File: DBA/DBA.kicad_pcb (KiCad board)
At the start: 2 copper layers, 45.7 x 61 mm, 3 parts, among them U1 ESP32_NodeMCU_v1.1

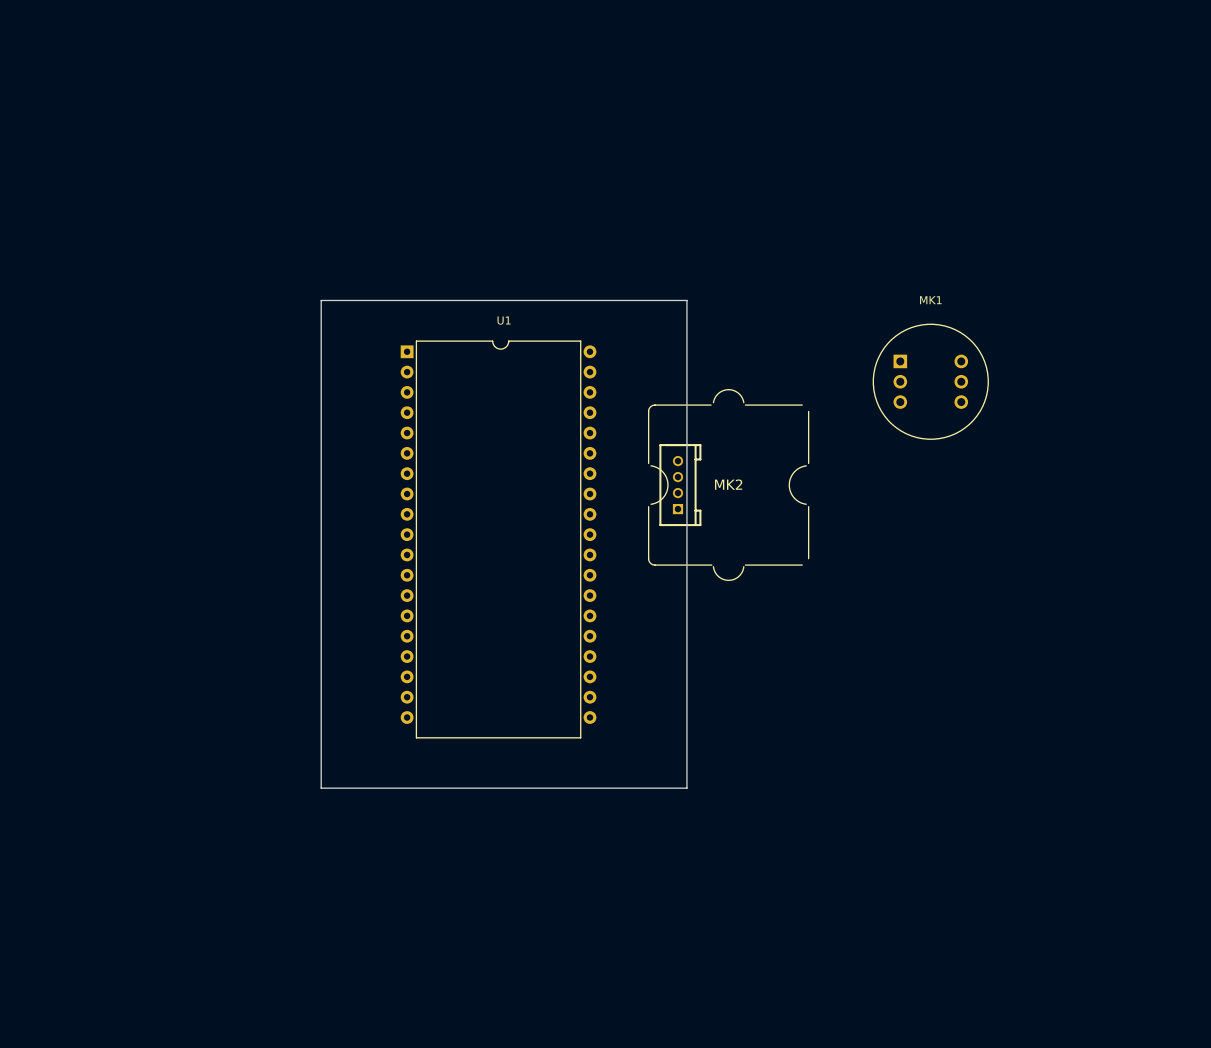
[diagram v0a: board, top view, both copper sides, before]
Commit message: First complete model
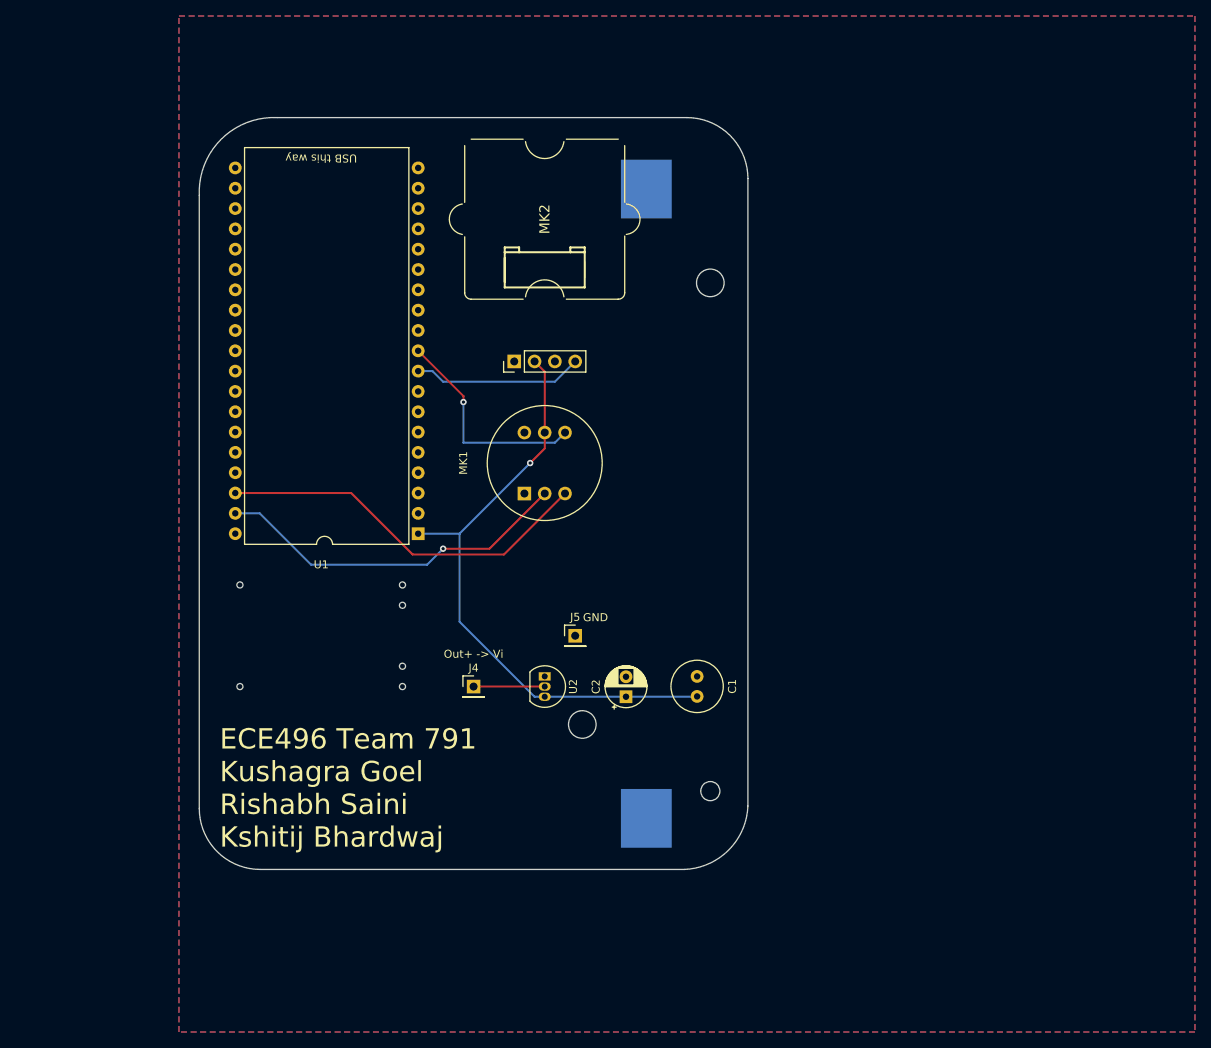
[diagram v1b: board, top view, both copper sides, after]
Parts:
- added A1: TP4056, custom:TP4056Board, B.Cu at (119.4, 101.6)
- added BT1: Battery_Cell, Battery:BatteryHolder_Keystone_1042_1x18650, B.Cu at (160.0, 86.4)
- added C1: 100n, Capacitor_THT:C_Radial_D6.3mm_H5.0mm_P2.50mm, F.Cu at (166.4, 108.0)
- added C2: 100u, Capacitor_THT:CP_Radial_D5.0mm_P2.50mm, F.Cu at (157.5, 110.5)
- added J4: Conn_01x01_Male, Connector_PinHeader_2.54mm:PinHeader_1x01_P2.54mm_Vertical, F.Cu at (138.4, 109.2)
- added J5: Conn_01x01_Male, Connector_PinHeader_2.54mm:PinHeader_1x01_P2.54mm_Vertical, F.Cu at (151.1, 102.9)
- added U2: MCP1700-3302E_TO92, Package_TO_SOT_THT:TO-92_Inline, F.Cu at (147.3, 108.0)
- moved MK1 49.3 mm to (147.3, 81.3), turned to 90 degrees
- moved MK2 40.4 mm to (147.3, 50.8), turned to 90 degrees
- moved U1 30.6 mm to (119.4, 68.6), turned to 180 degrees
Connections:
- MK2 pad 4: unconnected-(MK2-Pad4) -> Net-(MK2-Pad4)
- U1 pad 9: unconnected-(U1-Pad9) -> Net-(MK2-Pad4)
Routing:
- net Net-(C1-Pad2): track 0.00 -> 76.2 mm, vias 0 -> 1
- net Net-(MK1-Pad3): track 0.00 -> 47.6 mm
- net Net-(MK1-Pad2): track 0.00 -> 45.0 mm, vias 0 -> 1
- net Net-(MK1-Pad4): track 0.00 -> 27.1 mm, vias 0 -> 1
- net Net-(MK2-Pad4): track 0.00 -> 21.2 mm
- net Net-(U2-Pad2): track 0.00 -> 8.89 mm
- added copper zone on B.Cu, net GND
- added copper zone on F.Cu, net GND
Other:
- board size 45.7 x 61 mm -> 68.6 x 94 mm
- board text added: "ECE496 Team 791 Kushagra Goel Rishabh Saini Kshitij Bhardwaj"

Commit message: first circular version{
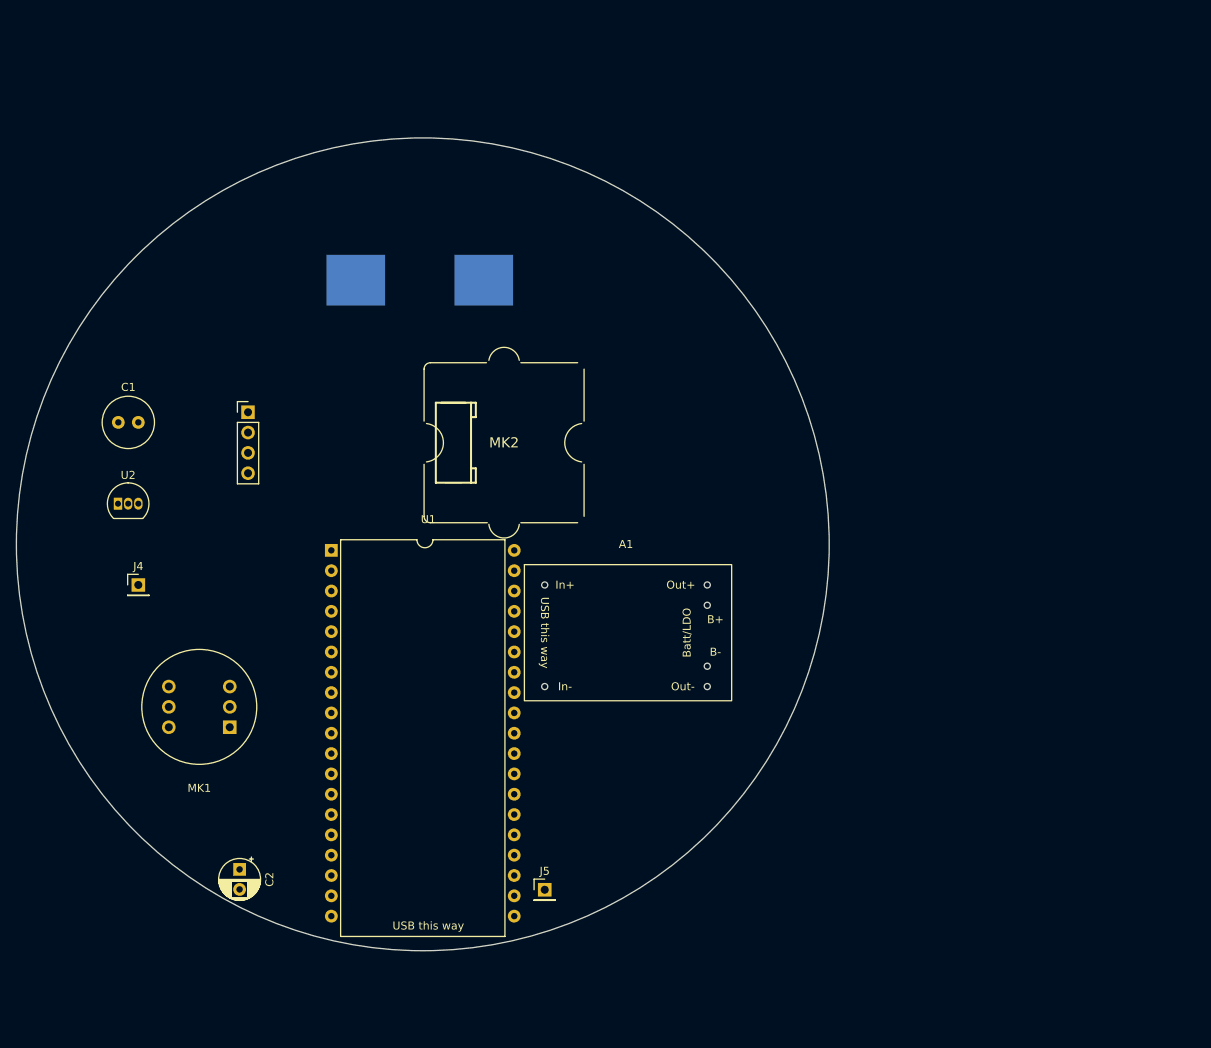
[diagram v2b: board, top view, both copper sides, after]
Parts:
- A1: moved to F.Cu
- BT1: footprint Battery:BatteryHolder_Keystone_1042_1x18650 -> Battery:Battery_Custom
- moved C1 79.0 mm to (94.0, 76.2), turned to 0 degrees
- moved U2 57.5 mm to (94.0, 86.4), turned to 0 degrees
- moved C2 52.9 mm to (109.2, 132.1), turned to -90 degrees
- moved MK1 52.9 mm to (104.1, 111.8), turned to 180 degrees
- moved U1 47.1 mm to (132.8, 113.7), turned to 0 degrees
- moved J4 43.8 mm to (96.5, 96.5)
- moved BT1 40.6 mm to (130.6, 58.4), turned to 180 degrees
- moved A1 38.2 mm to (157.5, 104.1)
- moved J5 32.0 mm to (147.3, 134.6)
- moved MK2 28.4 mm to (142.2, 78.7), turned to 0 degrees
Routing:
- net Net-(C1-Pad2): track 76.2 -> 0.00 mm, vias 1 -> 0
- net Net-(MK1-Pad3): track 47.6 -> 0.00 mm
- net Net-(MK1-Pad2): track 45.0 -> 0.00 mm, vias 1 -> 0
- net Net-(MK1-Pad4): track 27.1 -> 0.00 mm, vias 1 -> 0
- net Net-(MK2-Pad4): track 21.2 -> 0.00 mm
- net Net-(J4-Pad1): track 8.89 -> 0.00 mm
- removed copper zone on B.Cu, net GND
- removed copper zone on F.Cu, net GND
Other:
- board size 68.6 x 94 mm -> 101.6 x 101.6 mm
- board text removed: "ECE496 Team 791 Kushagra Goel Rishabh Saini Kshitij Bhardwaj"

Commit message: Final circular design
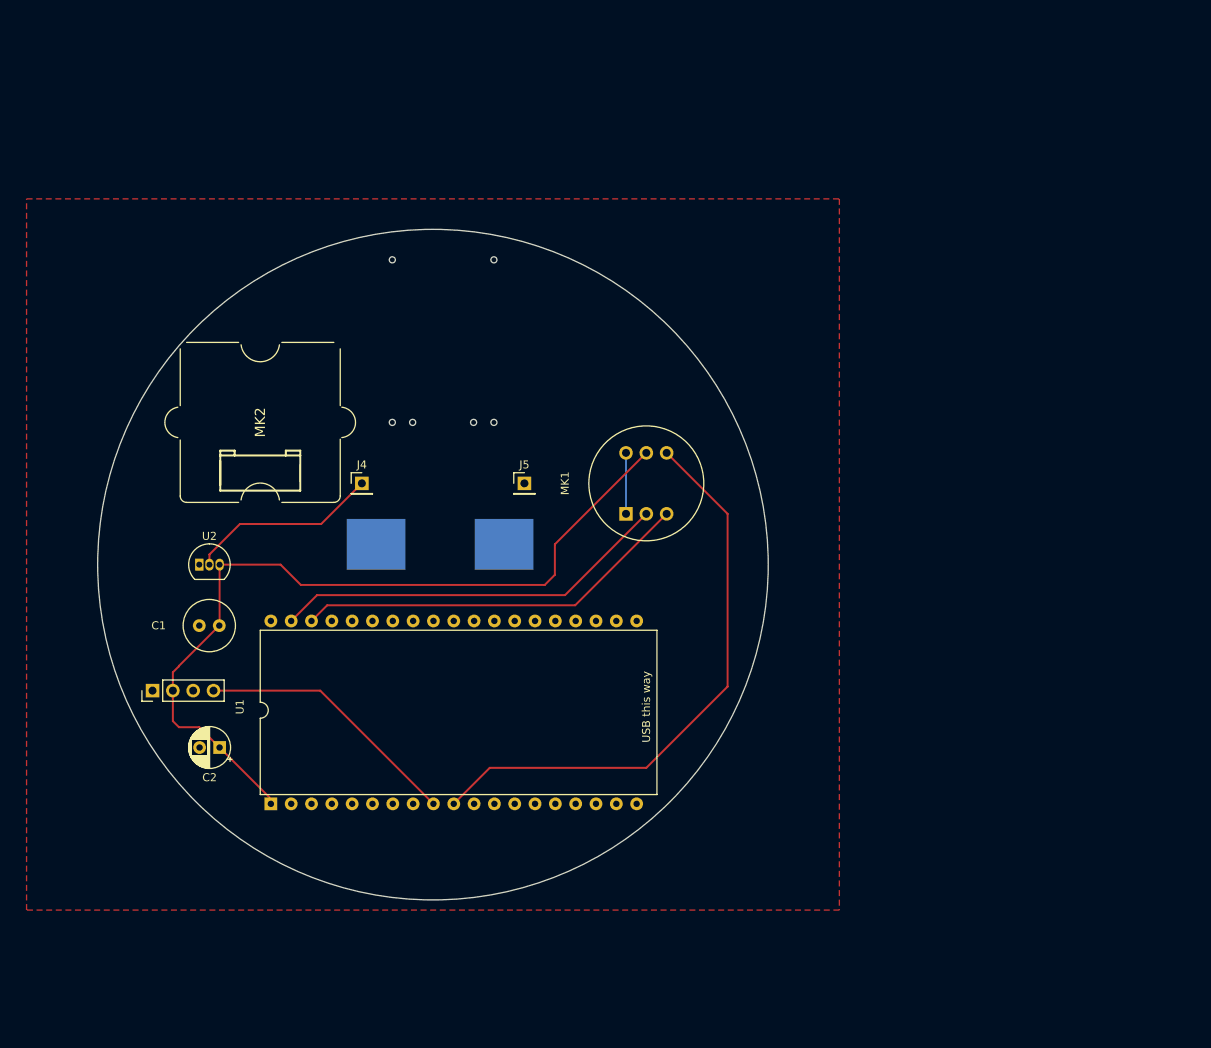
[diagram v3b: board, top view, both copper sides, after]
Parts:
- A1: moved to B.Cu
- moved MK1 62.5 mm to (160.0, 83.8), turned to 90 degrees
- moved J5 50.9 mm to (144.8, 83.8)
- moved A1 43.8 mm to (135.9, 66.0), turned to -90 degrees
- moved BT1 33.4 mm to (135.4, 91.4), turned to 0 degrees
- moved J4 30.7 mm to (124.5, 83.8)
- moved MK2 30.6 mm to (111.8, 76.2), turned to 90 degrees
- moved C1 27.3 mm to (104.1, 101.6)
- moved C2 15.4 mm to (106.7, 116.8), turned to 180 degrees
- moved U2 12.7 mm to (104.1, 94.0)
- moved U1 2.70 mm to (134.6, 111.8), turned to 90 degrees
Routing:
- net Net-(C1-Pad2): track 0.00 -> 102.3 mm
- net Net-(MK1-Pad4): track 0.00 -> 72.7 mm
- net Net-(MK1-Pad2): track 0.00 -> 49.9 mm
- net Net-(MK1-Pad3): track 0.00 -> 49.9 mm
- net Net-(MK2-Pad4): track 0.00 -> 33.4 mm
- net Net-(J4-Pad1): track 0.00 -> 24.0 mm
- net GND: track 0.00 -> 7.62 mm
- added copper zone on F.Cu, net GND
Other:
- board size 101.6 x 101.6 mm -> 83.8 x 83.8 mm
